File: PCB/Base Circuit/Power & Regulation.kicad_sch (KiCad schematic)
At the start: 24 parts, among them Q1_REVERSE PMOS, SW1_ESTOP SW_SPST

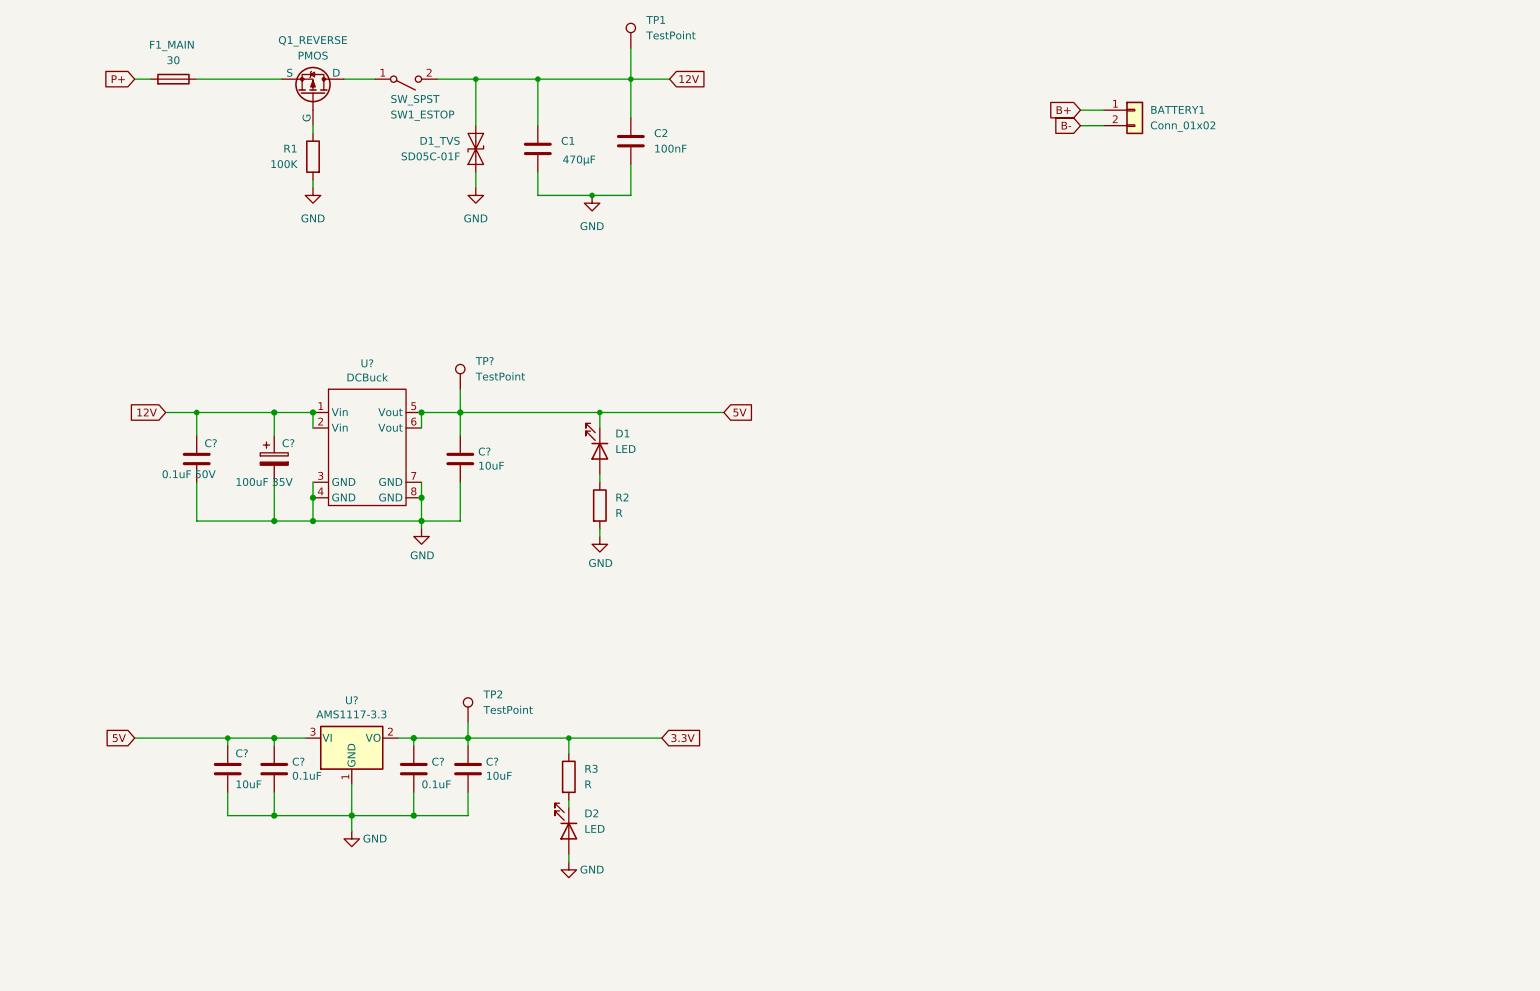
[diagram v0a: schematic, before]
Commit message: PCB Updated
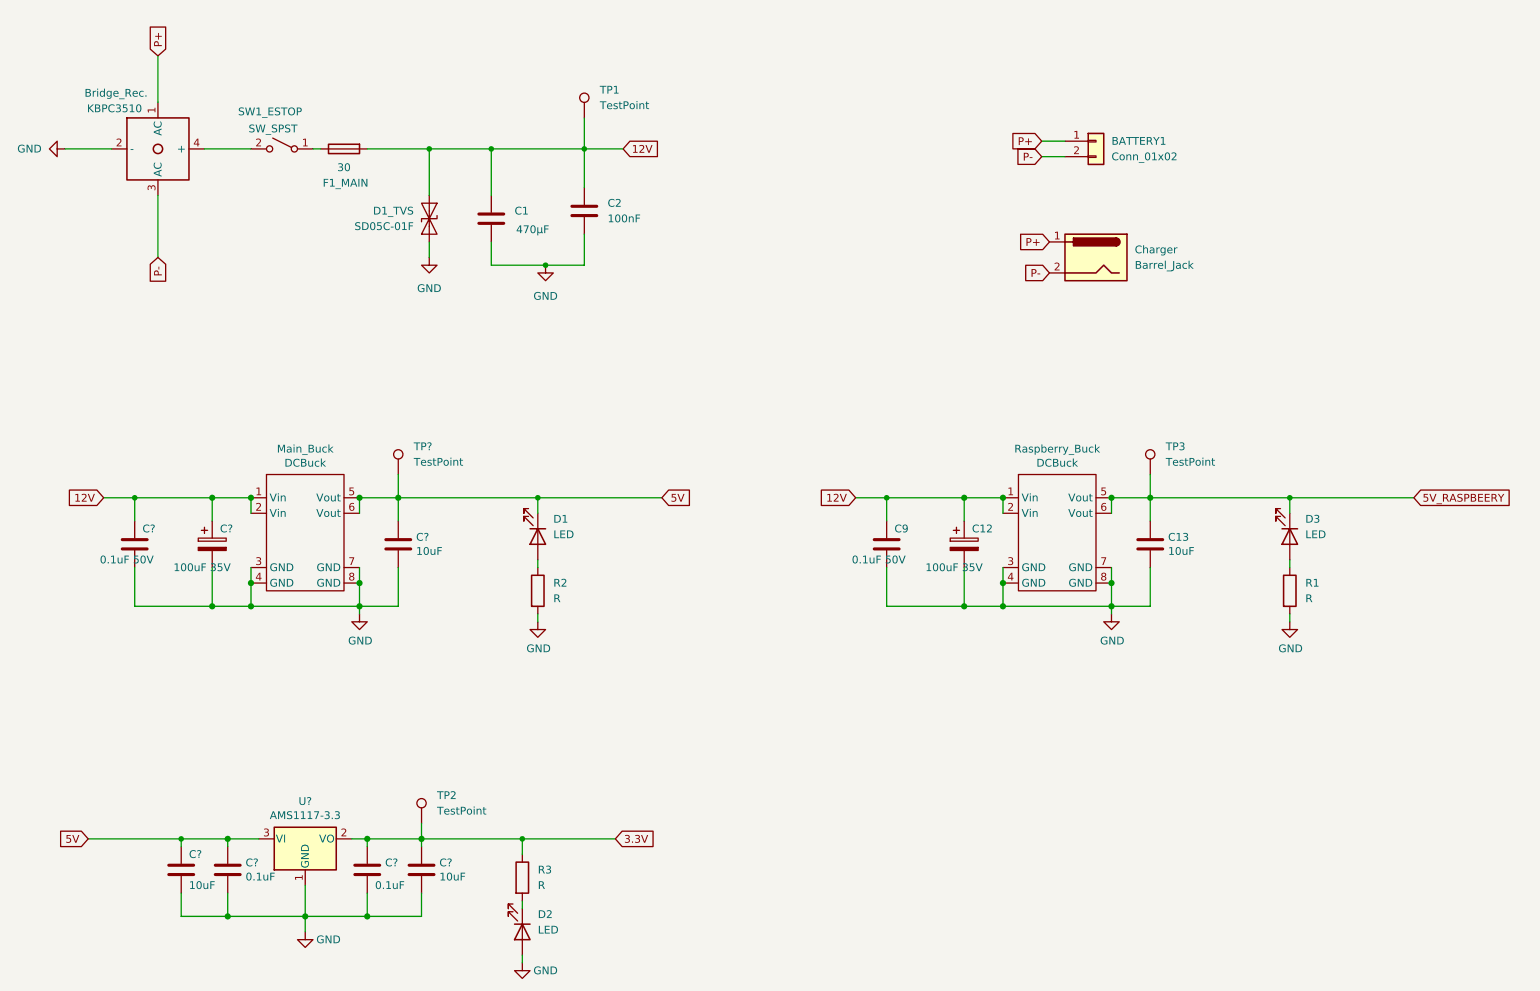
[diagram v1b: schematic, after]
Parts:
- removed Q1_REVERSE: PMOS, symbol Simulation_SPICE:PMOS
- added Bridge_Rec.: KBPC3510, symbol New_Library:KBPC3510
- added C12: 100uF 35V, Capacitor_SMD:CP_Elec_6.3x7.7, symbol Device:CP
- added C13: 10uF, PrntrBoardV2:C_0603_1608Metric, symbol Device:C
- added C9: 0.1uF 50V, PrntrBoardV2:C_0603_1608Metric, symbol Device:C
- added Charger: Barrel_Jack, symbol Connector:Barrel_Jack
- added D3: LED, symbol Device:LED
- added Raspberry_Buck: DCBuck, PrntrBoardV2:Buck2217, symbol BuckConverter:DCBuck
- added TP3: TestPoint, symbol Connector:TestPoint
- R1: value 100K -> R
- gave numbers to parts that had none: 1
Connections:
- net B+ is gone; now on net P+: BATTERY1.1 (Pin_1)
- net 12V: now also F1_MAIN.2, C12.1, C9.1, Raspberry_Buck.1 (Vin), Raspberry_Buck.2 (Vin); no longer SW1_ESTOP.2 (B)
- net GND: now also Bridge_Rec..2 (-), C12.2, C13.2, C9.2, Raspberry_Buck.3 (GND), Raspberry_Buck.4 (GND), Raspberry_Buck.7 (GND), Raspberry_Buck.8 (GND)
- net P+: now also Bridge_Rec..1 (AC), Charger.1; no longer F1_MAIN.2
- net at SW1_ESTOP.1 (A): now also F1_MAIN.1
- net at R1.1: now also D3.2 (A)
- net B- renamed P-
- net P-: now also Bridge_Rec..3 (AC), Charger.2
- new net: Bridge_Rec..4 (+), SW1_ESTOP.2 (B)
- new net 5V_RASPBEERY: C13.1, D3.1 (K), Raspberry_Buck.5 (Vout), Raspberry_Buck.6 (Vout), TP3.1
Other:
- moved on the sheet: BATTERY1, C1, C2, C?, D1, D1_TVS, D2, F1_MAIN, Main_Buck, R2, R3, SW1_ESTOP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
